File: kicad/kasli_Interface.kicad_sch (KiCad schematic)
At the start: 40 parts, among them J2 N2530-6002-RB, U14 SN65MLVD040RGZT, U15 SN65MLVD040RGZT, U16 24AA02E48T-I/OT

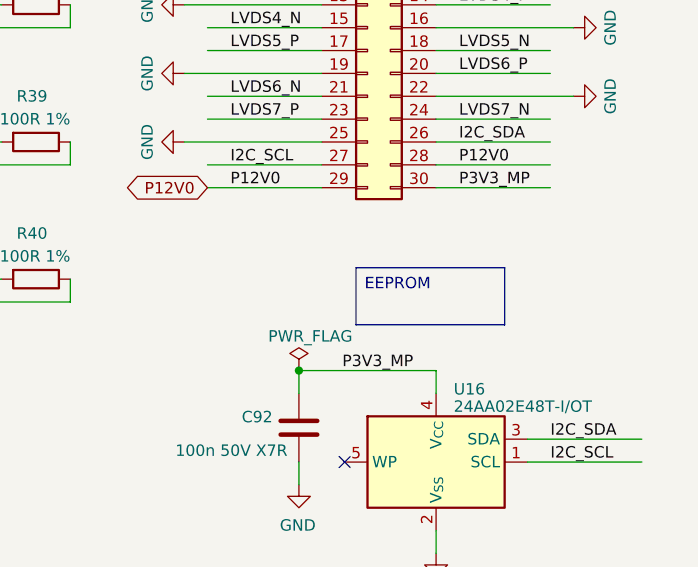
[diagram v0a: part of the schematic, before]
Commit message: kicad updated
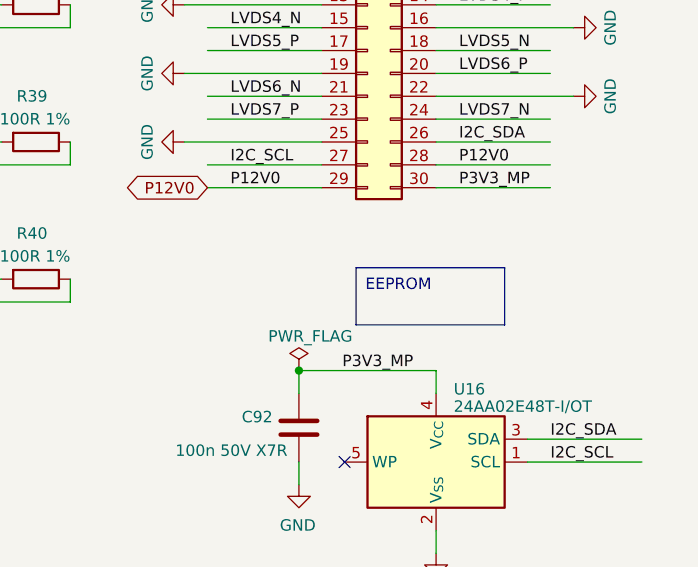
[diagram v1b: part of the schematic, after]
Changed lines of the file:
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@@
 (kicad_sch
-	(version 20250114)
+	(version 20231120)
 	(generator "eeschema")
-	(generator_version "9.0")
+	(generator_version "8.0")
 	(paper "A4")
-	(text_box "EEPROM\n"
-		(exclude_from_sim no)
-		(at 244.475 71.12 0)
-		(size 16.51 6.35)
-		(margins 0.9525 0.9525 0.9525 0.9525)
-		(stroke
-			(width 0)
-			(type default)
-			(color 0 0 0 1)
-		)
-		(fill
-			(type color)
-			(color 255 255 150 1)
-		)
-		(effects
-			(font
-				(size 1.27 1.27)
-			)
-			(justify left top)
-		)
-	)
 	(junction
 		(at 42.545 173.99)
@@
 		)
 	)
+	(text_box "EEPROM\n"
+		(exclude_from_sim no)
+		(at 244.475 71.12 0)
+		(size 16.51 6.35)
+		(stroke
+			(width 0)
+			(type default)
+			(color 0 0 0 1)
+		)
+		(fill
+			(type color)
+			(color 255 255 150 1)
+		)
+		(effects
+			(font
+				(size 1.27 1.27)
+			)
+			(justify left top)
+		)
+	)
